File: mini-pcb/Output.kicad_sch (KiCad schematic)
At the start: 15 parts, among them U2 OPA1664D

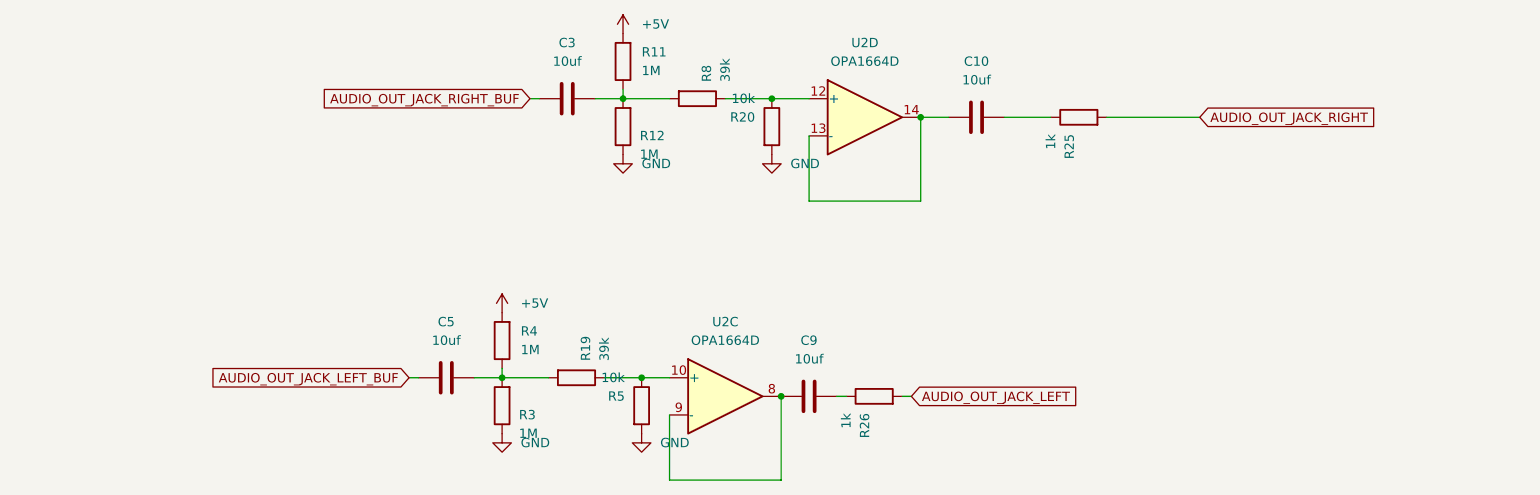
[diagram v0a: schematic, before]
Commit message: ordered pcb
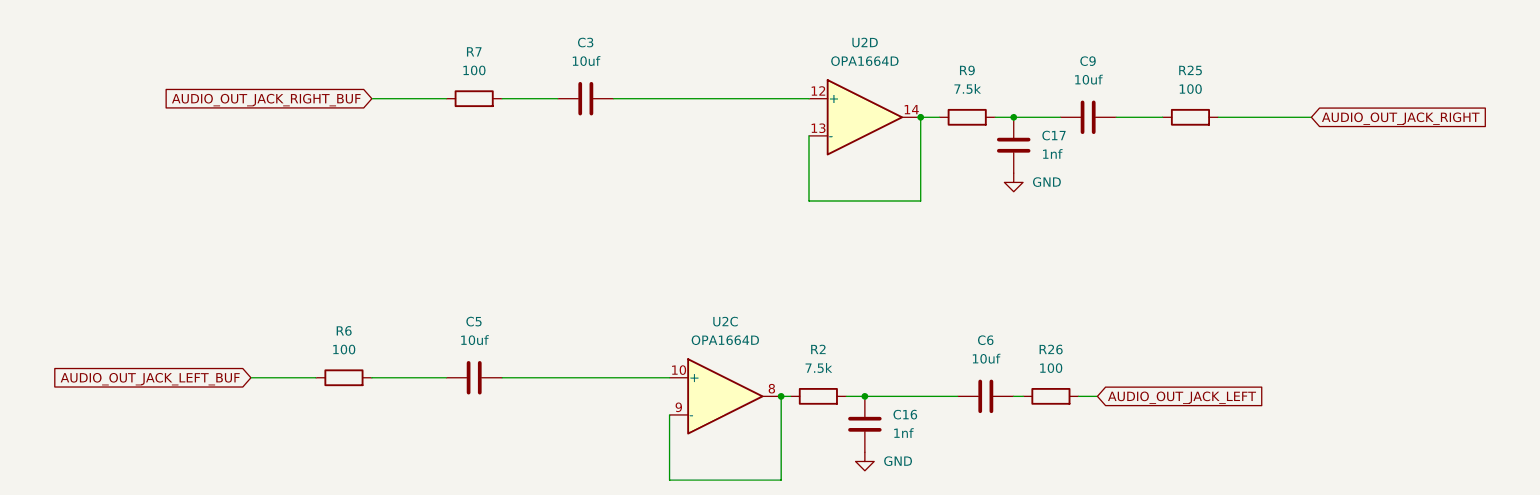
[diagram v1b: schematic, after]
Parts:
- removed C10: 10uf, Capacitor_SMD:C_0805_2012Metric, symbol Device:C
- removed R11, R12, R3, R4: 1M, Resistor_SMD:R_0603_1608Metric, symbol Device:R
- removed R19, R8: 39k, Resistor_SMD:R_0603_1608Metric, symbol Device:R
- removed R20, R5: 10k, Resistor_SMD:R_0603_1608Metric, symbol Device:R
- added C16, C17: 1nf, Capacitor_SMD:C_0805_2012Metric, symbol Device:C
- added C6: 10uf, Capacitor_SMD:C_0805_2012Metric, symbol Device:C
- added R2, R9: 7.5k, Resistor_SMD:R_0603_1608Metric, symbol Device:R
- added R6, R7: 100, Resistor_SMD:R_0603_1608Metric, symbol Device:R
- C3, C5, C9: MPN (none) -> C440198
- R25, R26: value 1k -> 100; MPN (none) -> C22775
- U2: MPN (none) -> C69414
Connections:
- net AUDIO_OUT_JACK_LEFT_BUF: now also R6.1; no longer C5.1
- net AUDIO_OUT_JACK_RIGHT_BUF: now also R7.1; no longer C3.1
- net GND: now also C16.1, C17.1
- net at U2.8, U2.9 (-): now also R2.1; no longer C9.1
- net at C9.2: now also R25.1; no longer R26.1
- net at C5.2: now also U2.10 (+)
- net at C3.2: now also U2.12 (+)
- net at U2.13 (-), U2.14: now also R9.1
- new net: C5.1, R6.2
- new net: C17.2, C9.1, R9.2
- new net: C6.2, R26.1
- new net: C3.1, R7.2
- new net: C16.2, C6.1, R2.2
